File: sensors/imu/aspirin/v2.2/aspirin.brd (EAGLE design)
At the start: 18.8 x 15.5 mm, 24 parts, among them IC1 LP2992, IC2 MS5611, IC3 >4KBIT SERIAL EEPROM HALF PRO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, U1 HMC5883, U2 MPU-6000

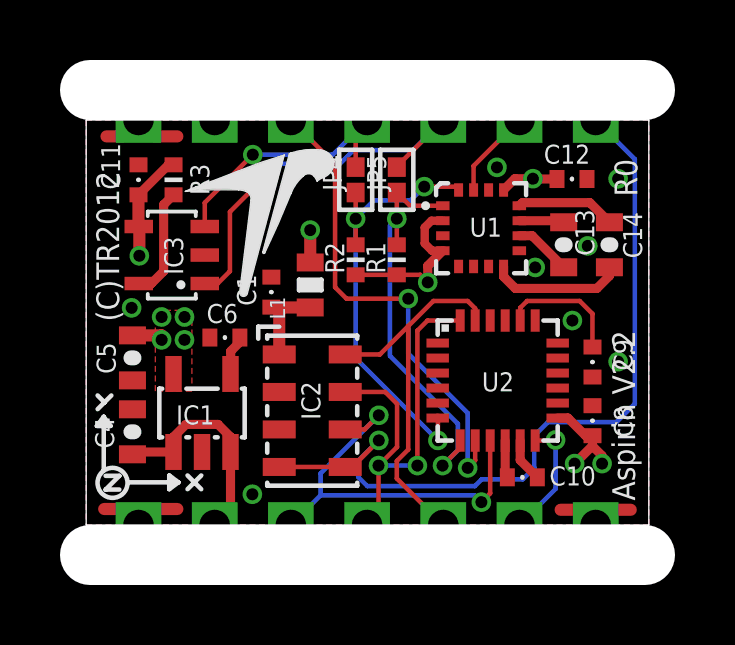
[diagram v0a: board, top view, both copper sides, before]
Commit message: Minor touchups.
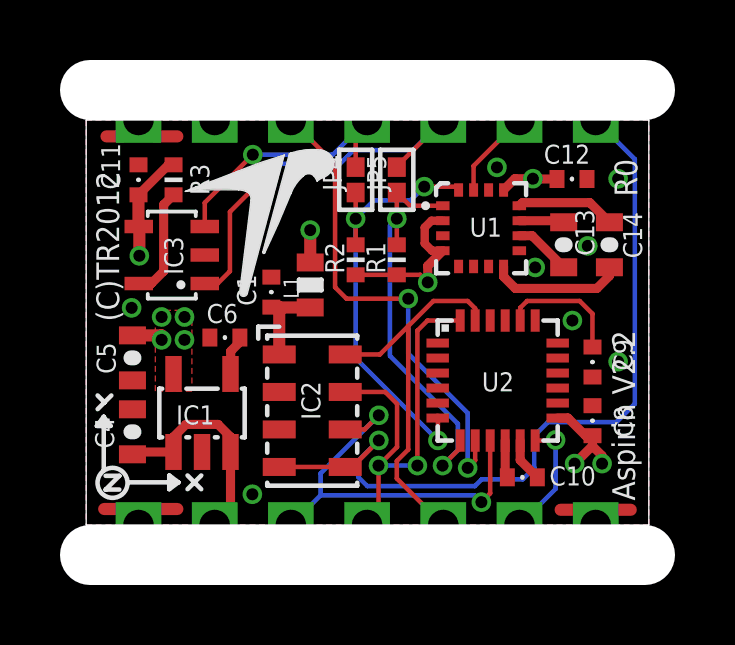
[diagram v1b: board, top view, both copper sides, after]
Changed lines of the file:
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@@
 <layer number="13" name="Route13" color="4" fill="5" visible="no" active="no"/>
 <layer number="14" name="Route14" color="1" fill="6" visible="no" active="no"/>
-<layer number="15" name="Route15" color="4" fill="6" visible="no" active="yes"/>
+<layer number="15" name="Route15" color="4" fill="6" visible="yes" active="yes"/>
 <layer number="16" name="Bottom" color="1" fill="1" visible="yes" active="yes"/>
 <layer number="17" name="Pads" color="2" fill="1" visible="yes" active="yes"/>
@@
 <layer number="44" name="Drills" color="7" fill="1" visible="no" active="yes"/>
 <layer number="45" name="Holes" color="7" fill="1" visible="no" active="yes"/>
-<layer number="46" name="Milling" color="3" fill="1" visible="no" active="yes"/>
+<layer number="46" name="Milling" color="3" fill="1" visible="yes" active="yes"/>
 <layer number="47" name="Measures" color="7" fill="1" visible="no" active="yes"/>
 <layer number="48" name="Document" color="7" fill="1" visible="no" active="yes"/>
@@
 <layer number="100" name="Muster" color="7" fill="1" visible="no" active="no"/>
 <layer number="101" name="Patch_Top" color="12" fill="4" visible="no" active="yes"/>
-<layer number="102" name="Vscore" color="7" fill="1" visible="no" active="yes"/>
+<layer number="102" name="Vscore" color="7" fill="1" visible="yes" active="yes"/>
 <layer number="103" name="origins2" color="7" fill="1" visible="no" active="yes"/>
 <layer number="104" name="Name" color="7" fill="1" visible="no" active="yes"/>
@@
 <attribute name="VALUE" x="4.2071" y="10.3632" size="0.635" layer="27" font="vector" ratio="16" rot="R90"/>
 </element>
-<element name="L1" library="res_cap" package="0603-IND" value="" x="7.4676" y="8.001" rot="R90">
-<attribute name="PARTNO" value="MMZ1608B601C" x="7.4676" y="8.001" size="1.778" layer="27" rot="R90" display="off"/>
+<element name="L1" library="res_cap" package="0603-IND" value="" x="7.4676" y="8.001" smashed="yes" rot="R90">
+<attribute name="PARTNO" value="ferrite-0603-600ohm" x="7.4676" y="8.001" size="1.778" layer="27" rot="R90" display="off"/>
+<attribute name="NAME" x="7.0866" y="7.5438" size="0.508" layer="25" font="vector" ratio="20" rot="R90"/>
+<attribute name="VALUE" x="8.763" y="6.858" size="0.508" layer="27" font="vector" ratio="20" rot="R90"/>
 </element>
 </elements>
@@
 </signal>
 </signals>
-<errors>
-</errors>
 </board>
 </drawing>
